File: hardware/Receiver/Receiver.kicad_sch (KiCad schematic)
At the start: 132 parts, among them J1 USB_C_Receptacle_USB2.0, J3 20021511-00006T4LF, J4 Conn_01x04, J6 JST_PH, Q1 2N7002, Q2 NMOS, Q3 NMOS, Q4 PMOS, SW1 Boot, SW1 Reset, SW3 1825027-8, U1 TPS22810DRV, U2 DMG6602SVTQ, U2 TPS22810DRV, U3 AZ1117-3.3, U3 DMG6602SVTQ, U4 TLV493DA1B6HTSA2, U8 ESP32-S3-MINI-1-N8

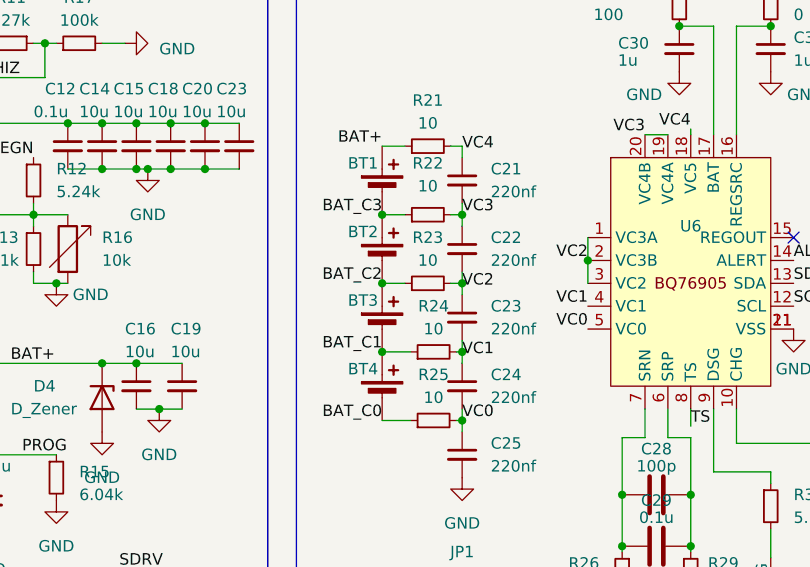
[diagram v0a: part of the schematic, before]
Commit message: update readme details
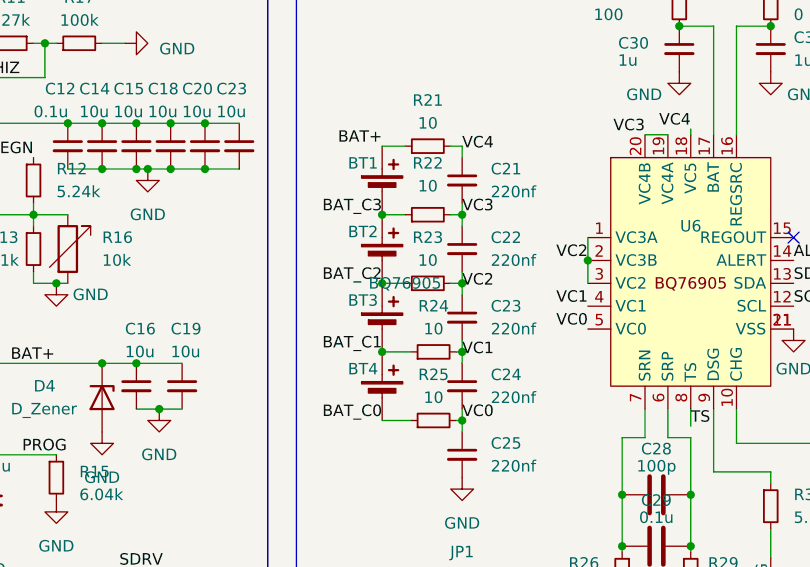
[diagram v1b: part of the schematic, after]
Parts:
- U6: value ~ -> BQ76905
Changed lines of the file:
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@@
       (effects (font (size 1.27 1.27)))
     )
-    (property "Value" "~" (at 134.62 144.145 0)
+    (property "Value" "BQ76905" (at 134.62 144.145 0)
       (effects (font (size 1.27 1.27)))
     )
